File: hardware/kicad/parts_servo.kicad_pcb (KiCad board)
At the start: 2 copper layers, 37.3 x 17.5 mm, 47 parts, among them Q110 NFET-DUAL, Q120 NFET-DUAL, U1 MCP1703-3302, U100 RT9625A, U200 AS5050, U50 NRF51822, X60 16MHz

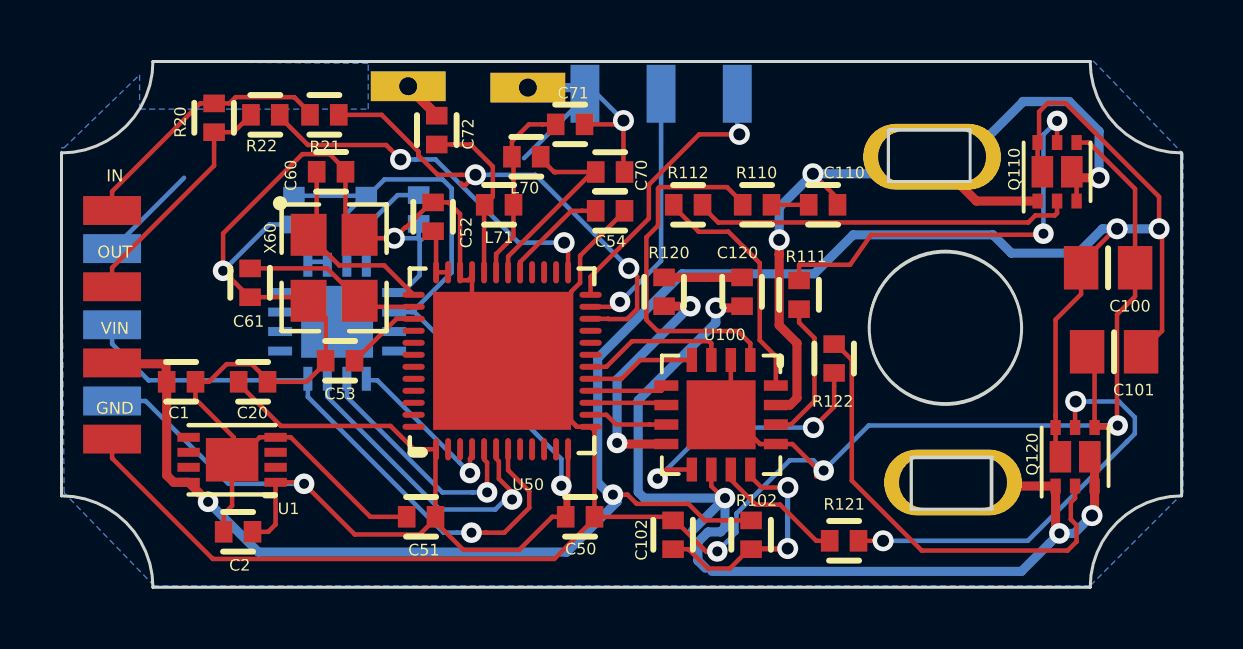
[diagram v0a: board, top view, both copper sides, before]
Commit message: board layout cleanup
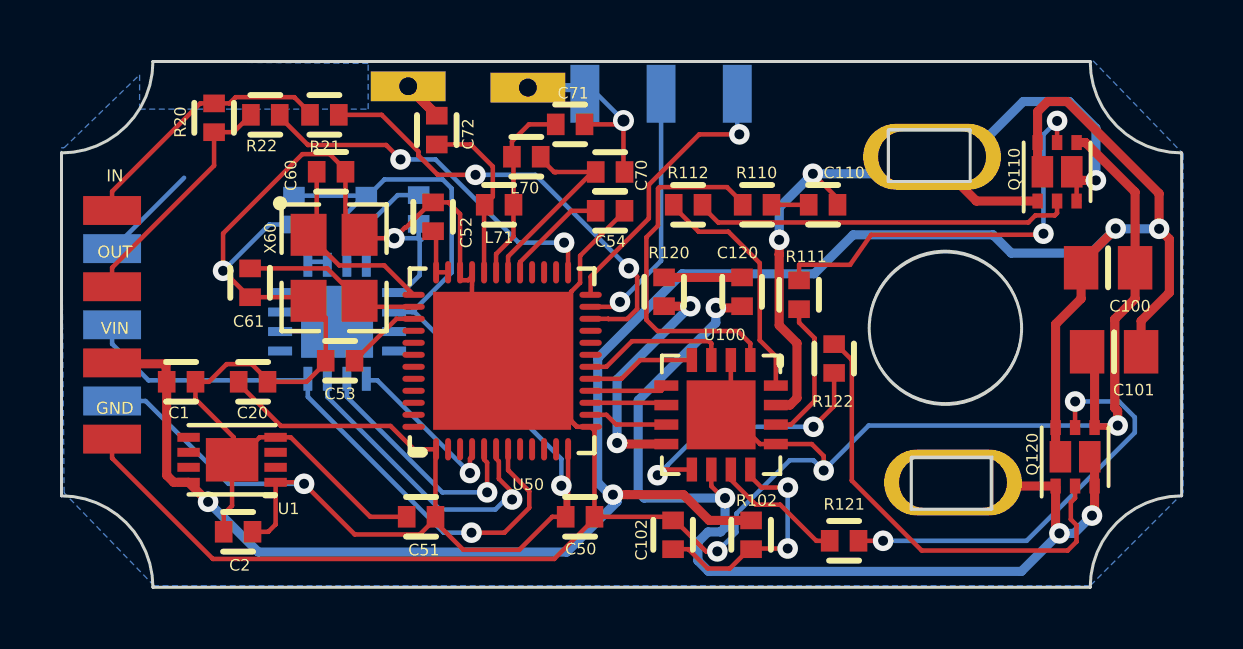
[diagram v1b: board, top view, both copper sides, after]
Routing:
- net Net-(C102-Pad1): track 11.3 -> 8.03 mm
- net /PWR_MotorA: track 39.1 -> 36.2 mm
- net GND: track 141.0 -> 143.5 mm
- net /PWR_MotorB: track 33.6 -> 32.5 mm
- net /UNIPOLAR_INPUT: track 15.7 -> 15.0 mm
